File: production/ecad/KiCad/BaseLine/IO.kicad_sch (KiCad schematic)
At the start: 1 part, among them U12 CD74HC4067M96

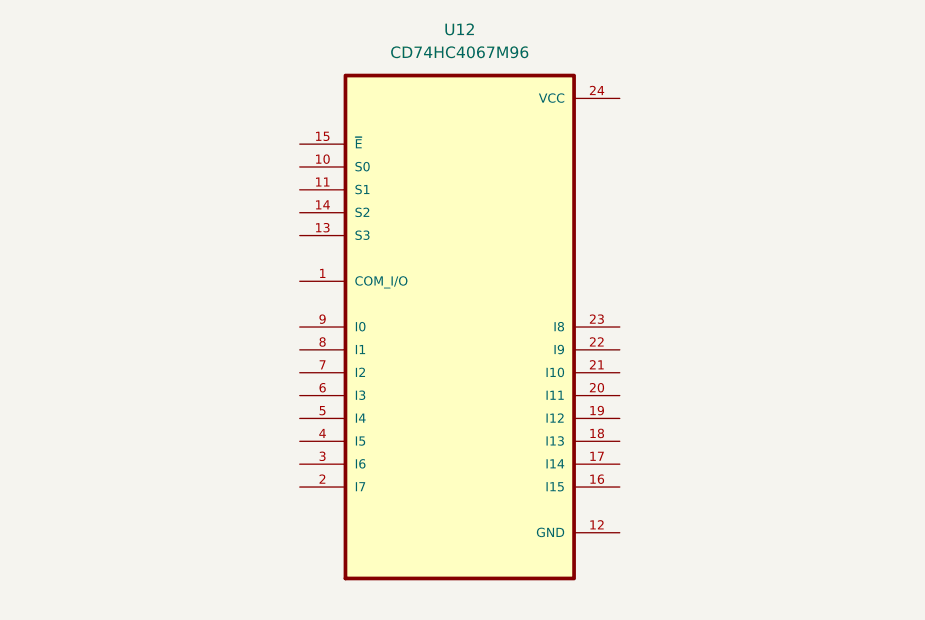
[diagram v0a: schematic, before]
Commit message: Update IO.kicad_sch
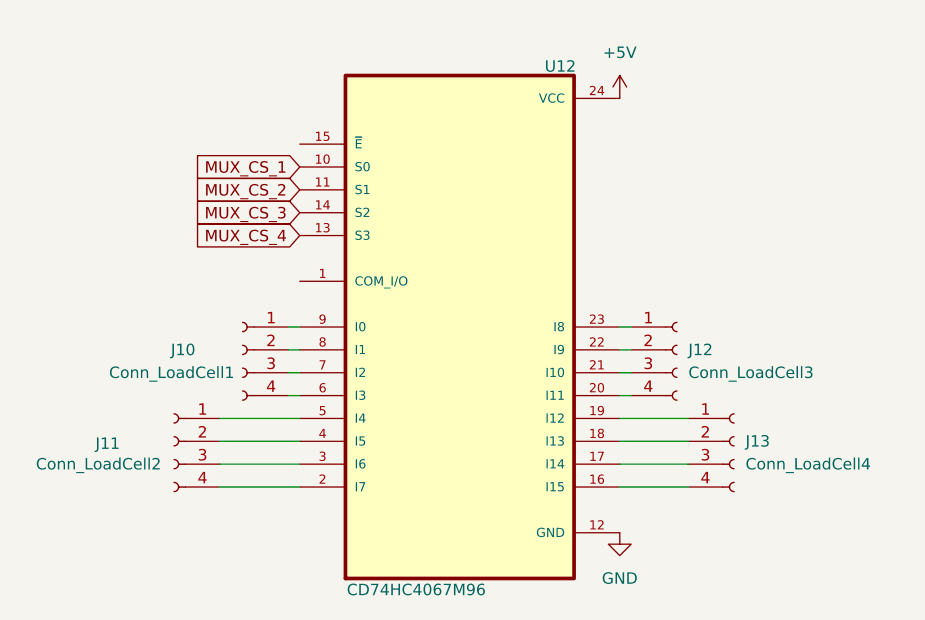
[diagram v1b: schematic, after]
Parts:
- added J10: Conn_LoadCell1, symbol Connector:Conn_01x04_Socket
- added J11: Conn_LoadCell2, symbol Connector:Conn_01x04_Socket
- added J12: Conn_LoadCell3, symbol Connector:Conn_01x04_Socket
- added J13: Conn_LoadCell4, symbol Connector:Conn_01x04_Socket
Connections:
- net MUX_CS_1: now reaches U12.10 (S0)
- net MUX_CS_2: now reaches U12.11 (S1)
- net GND: now reaches U12.12 (GND)
- net MUX_CS_4: now reaches U12.13 (S3)
- net MUX_CS_3: now reaches U12.14 (S2)
- net at U12.16 (I15): now also J13.4 (Pin_4)
- net at U12.17 (I14): now also J13.3 (Pin_3)
- net at U12.18 (I13): now also J13.2 (Pin_2)
- net at U12.19 (I12): now also J13.1 (Pin_1)
- net at U12.2 (I7): now also J11.4 (Pin_4)
- net at U12.20 (I11): now also J12.4 (Pin_4)
- net at U12.21 (I10): now also J12.3 (Pin_3)
- net at U12.22 (I9): now also J12.2 (Pin_2)
- net at U12.23 (I8): now also J12.1 (Pin_1)
- net +5V: now reaches U12.24 (VCC)
- net at U12.3 (I6): now also J11.3 (Pin_3)
- net at U12.4 (I5): now also J11.2 (Pin_2)
- net at U12.5 (I4): now also J11.1 (Pin_1)
- net at U12.6 (I3): now also J10.4 (Pin_4)
- net at U12.7 (I2): now also J10.3 (Pin_3)
- net at U12.8 (I1): now also J10.2 (Pin_2)
- net at U12.9 (I0): now also J10.1 (Pin_1)
